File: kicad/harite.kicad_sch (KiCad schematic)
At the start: 77 parts, among them J1 503480-0500, J4 5034801200, J5 5034801200, U1 RP2040_Zero, U2 RP2040_Zero

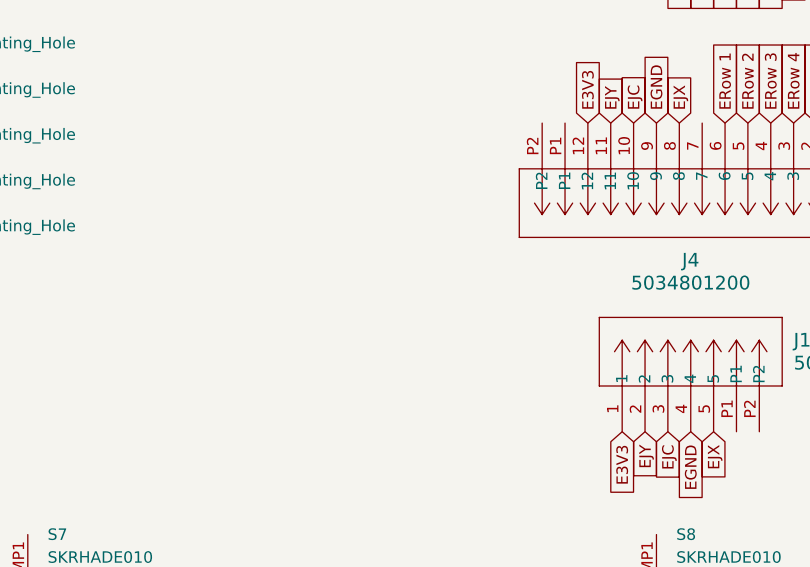
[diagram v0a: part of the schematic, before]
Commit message: update
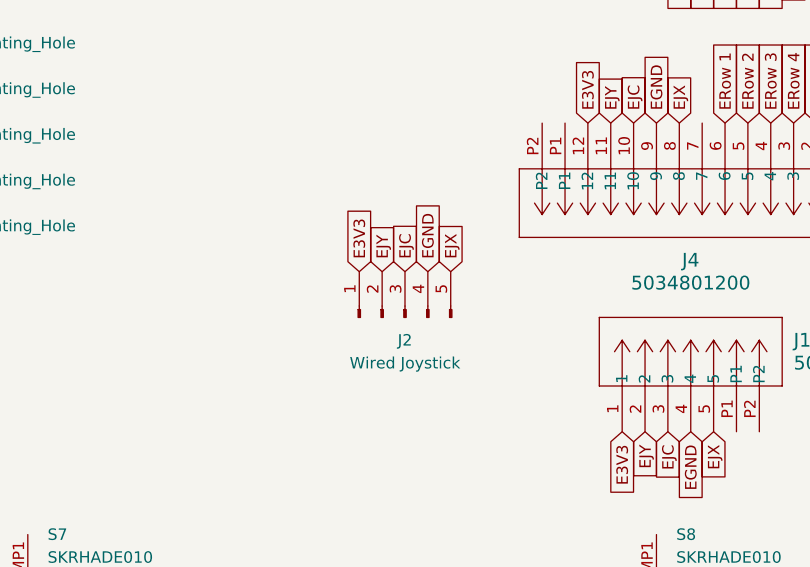
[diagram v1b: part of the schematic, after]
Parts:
- added J2: Wired Joystick, Wired-Joystick, symbol Connector:Conn_01x05_Pin
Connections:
- net E3V3: now also J2.1 (Pin_1)
- net EGND: now also J2.4 (Pin_4)
- net EJC: now also J2.3 (Pin_3)
- net EJX: now also J2.5 (Pin_5)
- net EJY: now also J2.2 (Pin_2)
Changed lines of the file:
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@@
 		)
 	)
+	(global_label "EJY"
+		(shape input)
+		(at 162.56 133.35 90)
+		(fields_autoplaced yes)
+		(effects
+			(font
+				(size 1.27 1.27)
+			)
+			(justify left)
+		)
+		(property "Intersheetrefs" "${INTERSHEET_REFS}"
+			(at 162.56 127.1596 90)
+			(effects
+				(font
+					(size 1.27 1.27)
+				)
+				(justify left)
+				(hide yes)
+			)
+		)
+	)
 	(global_label "RCol 3"
 		(shape input)
@@
 		)
 	)
+	(global_label "E3V3"
+		(shape input)
+		(at 160.02 133.35 90)
+		(fields_autoplaced yes)
+		(effects
+			(font
+				(size 1.27 1.27)
+			)
+			(justify left)
+		)
+		(property "Intersheetrefs" "${INTERSHEET_REFS}"
+			(at 160.02 125.7082 90)
+			(effects
+				(font
+					(size 1.27 1.27)
+				)
+				(justify left)
+				(hide yes)
+			)
+		)
+	)
 	(global_label "JX"
 		(shape input)
@@
 		)
 	)
+	(global_label "EJC"
+		(shape input)
+		(at 165.1 133.35 90)
+		(fields_autoplaced yes)
+		(effects
+			(font
+				(size 1.27 1.27)
+			)
+			(justify left)
+		)
+		(property "Intersheetrefs" "${INTERSHEET_REFS}"
+			(at 165.1 126.9782 90)
+			(effects
+				(font
+					(size 1.27 1.27)
+				)
+				(justify left)
+				(hide yes)
+			)
+		)
+	)
 	(global_label "JC"
 		(shape input)
@@
 		)
 	)
+	(global_label "EJX"
+		(shape input)
+		(at 170.18 133.35 90)
+		(fields_autoplaced yes)
+		(effects
+			(font
+				(size 1.27 1.27)
+			)
+			(justify left)
+		)
+		(property "Intersheetrefs" "${INTERSHEET_REFS}"
+			(at 170.18 127.0387 90)
+			(effects
+				(font
+					(size 1.27 1.27)
+				)
+				(justify left)
+				(hide yes)
+			)
+		)
+	)
 	(global_label "Col 3"
 		(shape input)
@@
 		)
 	)
+	(global_label "EGND"
+		(shape input)
+		(at 167.64 133.35 90)
+		(fields_autoplaced yes)
+		(effects
+			(font
+				(size 1.27 1.27)
+			)
+			(justify left)
+		)
+		(property "Intersheetrefs" "${INTERSHEET_REFS}"
+			(at 167.64 125.3453 90)
+			(effects
+				(font
+					(size 1.27 1.27)
+				)
+				(justify left)
+				(hide yes)
+			)
+		)
+	)
 	(global_label "Row 5"
 		(shape input)
@@
 					(unit 1)
 				)
+			)
+		)
+	)
+	(symbol
+		(lib_id "Connector:Conn_01x05_Pin")
+		(at 165.1 138.43 90)
+		(unit 1)
+		(exclude_from_sim no)
+		(in_bom yes)
+		(on_board yes)
+		(dnp no)
+		(fields_autoplaced yes)
+		(property "Reference" "J2"
+			(at 165.1 140.97 90)
+			(effects
+				(font
+					(size 1.27 1.27)
+				)
+			)
+		)
+		(property "Value" "Wired Joystick"
+			(at 165.1 143.51 90)
+			(effects
+				(font
+					(size 1.27 1.27)
+				)
+			)
+		)
+		(property "Footprint" "Wired-Joystick"
+			(at 165.1 138.43 0)
+			(effects
+				(font
+					(size 1.27 1.27)
+				)
+				(hide yes)
+			)
+		)
+		(property "Datasheet" "~"
+			(at 165.1 138.43 0)
+			(effects
+				(font
+					(size 1.27 1.27)
+				)
+				(hide yes)
+			)
+		)
+		(property "Description" "Generic connector, single row, 01x05, script generated"
+			(at 165.1 138.43 0)
+			(effects
+				(font
+					(size 1.27 1.27)
+				)
+				(hide yes)
+			)
+		)
+		(pin "4"
+		)
+		(pin "3"
+		)
+		(pin "2"
+		)
+		(pin "1"
+		)
+		(pin "5"
+		)
+		(instances
+			(project "harite"
+				(path "/feb70c3f-3e34-4f8f-9694-07d231f2d237"
+					(reference "J2")
+					(unit 1)
+				)

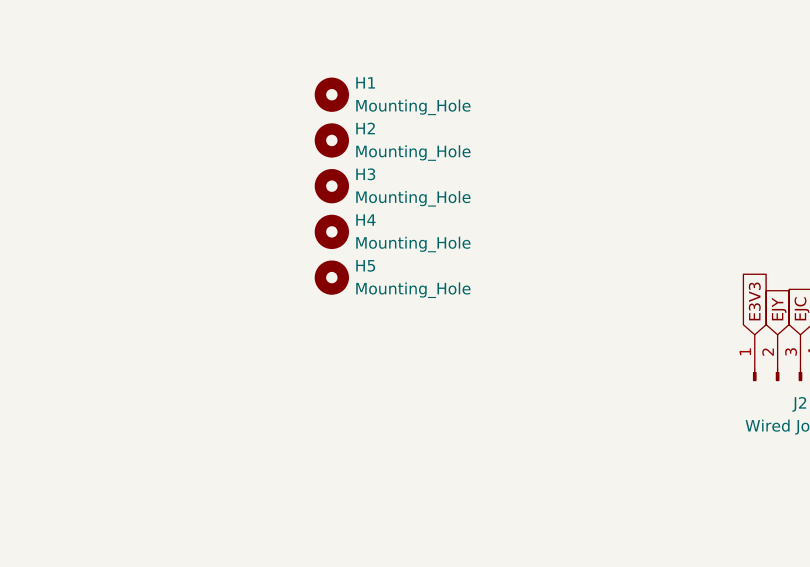
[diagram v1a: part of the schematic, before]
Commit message: add joycon
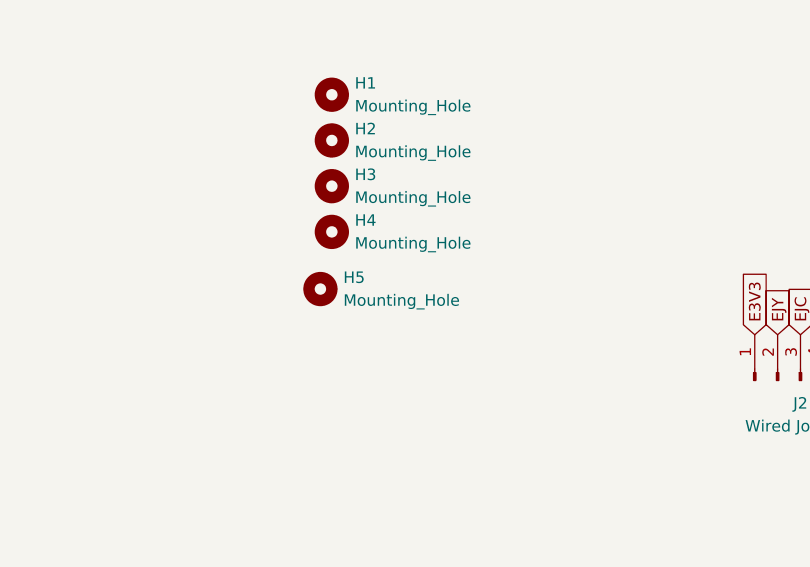
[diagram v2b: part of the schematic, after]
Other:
- moved on the sheet: H5
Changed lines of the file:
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@@
 	(symbol
 		(lib_id "ScottoKeebs:Placeholder_Mounting_Hole")
-		(at 113.03 127 0)
+		(at 111.76 128.27 0)
 		(unit 1)
 		(exclude_from_sim no)
@@
 		(fields_autoplaced yes)
 		(property "Reference" "H5"
-			(at 115.57 125.7299 0)
+			(at 114.3 126.9999 0)
 			(effects
 				(font
@@
 		)
 		(property "Value" "Mounting_Hole"
-			(at 115.57 128.2699 0)
+			(at 114.3 129.5399 0)
 			(effects
 				(font
@@
 		)
 		(property "Footprint" "MountingHole:MountingHole_2.2mm_M2_Pad_Via"
-			(at 113.03 127 0)
+			(at 111.76 128.27 0)
 			(effects
 				(font
@@
 		)
 		(property "Datasheet" "~"
-			(at 113.03 127 0)
+			(at 111.76 128.27 0)
 			(effects
 				(font
@@
 		)
 		(property "Description" "Mounting Hole without connection"
-			(at 113.03 127 0)
+			(at 111.76 128.27 0)
 			(effects
 				(font
@@
 	)
 	(symbol
-		(lib_id "ScottoKeebs:Placeholder_Mounting_Hole")
-		(at 120.65 243.84 0)
-		(unit 1)
-		(exclude_from_sim no)
-		(in_bom yes)
-		(on_board yes)
-		(dnp no)
-		(fields_autoplaced yes)
-		(property "Reference" "H9"
-			(at 123.19 242.5699 0)
-			(effects
-				(font
-					(size 1.27 1.27)
-				)
-				(justify left)
-			)
-		)
-		(property "Value" "Mounting_Hole"
-			(at 123.19 245.1099 0)
-			(effects
-				(font
-					(size 1.27 1.27)
-				)
-				(justify left)
-			)
-		)
-		(property "Footprint" "MountingHole:MountingHole_2.2mm_M2_Pad_Via"
-			(at 120.65 243.84 0)
-			(effects
-				(font
-					(size 1.27 1.27)
-				)
-				(hide yes)
-			)
-		)
-		(property "Datasheet" "~"
-			(at 120.65 243.84 0)
-			(effects
-				(font
-					(size 1.27 1.27)
-				)
-				(hide yes)
-			)
-		)
-		(property "Description" "Mounting Hole without connection"
-			(at 120.65 243.84 0)
-			(effects
-				(font
-					(size 1.27 1.27)
-				)
-				(hide yes)
-			)
-		)
-		(instances
-			(project "harite"
-				(path "/feb70c3f-3e34-4f8f-9694-07d231f2d237"
-					(reference "H9")
-					(unit 1)
-				)
-			)
-		)
-	)
-	(symbol
 		(lib_id "Device:D")
 		(at 163.83 60.96 0)
@@
 	)
 	(symbol
-		(lib_id "ScottoKeebs:Placeholder_Mounting_Hole")
-		(at 120.65 248.92 0)
-		(unit 1)
-		(exclude_from_sim no)
-		(in_bom yes)
-		(on_board yes)
-		(dnp no)
-		(fields_autoplaced yes)
-		(property "Reference" "H10"
-			(at 123.19 247.6499 0)
-			(effects
-				(font
-					(size 1.27 1.27)
-				)
-				(justify left)
-			)
-		)
-		(property "Value" "Mounting_Hole"
-			(at 123.19 250.1899 0)
-			(effects
-				(font
-					(size 1.27 1.27)
-				)
-				(justify left)
-			)
-		)
-		(property "Footprint" "MountingHole:MountingHole_2.2mm_M2_Pad_Via"
-			(at 120.65 248.92 0)
-			(effects
-				(font
-					(size 1.27 1.27)
-				)
-				(hide yes)
-			)
-		)
-		(property "Datasheet" "~"
-			(at 120.65 248.92 0)
-			(effects
-				(font
-					(size 1.27 1.27)
-				)
-				(hide yes)
-			)
-		)
-		(property "Description" "Mounting Hole without connection"
-			(at 120.65 248.92 0)
-			(effects
-				(font
-					(size 1.27 1.27)
-				)
-				(hide yes)
-			)
-		)
-		(instances
-			(project "harite"
-				(path "/feb70c3f-3e34-4f8f-9694-07d231f2d237"
-					(reference "H10")
-					(unit 1)
-				)
-			)
-		)
-	)
-	(symbol
 		(lib_id "Device:D")
 		(at 276.86 60.96 180)
@@
 	)
 	(symbol
+		(lib_id "ScottoKeebs:Placeholder_Mounting_Hole")
+		(at 120.65 243.84 0)
+		(unit 1)
+		(exclude_from_sim no)
+		(in_bom yes)
+		(on_board yes)
+		(dnp no)
+		(fields_autoplaced yes)
+		(property "Reference" "H9"
+			(at 123.19 242.5699 0)
+			(effects
+				(font
+					(size 1.27 1.27)
+				)
+				(justify left)
+			)
+		)
+		(property "Value" "Mounting_Hole"
+			(at 123.19 245.1099 0)
+			(effects
+				(font
+					(size 1.27 1.27)
+				)
+				(justify left)
+			)
+		)
+		(property "Footprint" "MountingHole:MountingHole_2.2mm_M2_Pad_Via"
+			(at 120.65 243.84 0)
+			(effects
+				(font
+					(size 1.27 1.27)
+				)
+				(hide yes)
+			)
+		)
+		(property "Datasheet" "~"
+			(at 120.65 243.84 0)
+			(effects
+				(font
+					(size 1.27 1.27)
+				)
+				(hide yes)
+			)
+		)
+		(property "Description" "Mounting Hole without connection"
+			(at 120.65 243.84 0)
+			(effects
+				(font
+					(size 1.27 1.27)
+				)
+				(hide yes)
+			)
+		)
+		(instances
+			(project "harite"
+				(path "/feb70c3f-3e34-4f8f-9694-07d231f2d237"
+					(reference "H9")
+					(unit 1)
+				)
+			)
+		)
+	)
+	(symbol
 		(lib_id "SKRHADE010:SKRHADE010")
 		(at 243.84 241.3 0)
@@
 					(unit 1)
 				)
+			)
+		)
+	)
+	(symbol
+		(lib_id "ScottoKeebs:Placeholder_Mounting_Hole")
+		(at 120.65 248.92 0)
+		(unit 1)
+		(exclude_from_sim no)
+		(in_bom yes)
+		(on_board yes)
+		(dnp no)
+		(fields_autoplaced yes)
+		(property "Reference" "H10"
+			(at 123.19 247.6499 0)
+			(effects
+				(font
+					(size 1.27 1.27)
+				)
+				(justify left)
+			)
+		)
+		(property "Value" "Mounting_Hole"
+			(at 123.19 250.1899 0)
+			(effects
+				(font
+					(size 1.27 1.27)
+				)
+				(justify left)
+			)
+		)
+		(property "Footprint" "MountingHole:MountingHole_2.2mm_M2_Pad_Via"
+			(at 120.65 248.92 0)
+			(effects
+				(font
+					(size 1.27 1.27)
+				)
+				(hide yes)
+			)
+		)
+		(property "Datasheet" "~"
+			(at 120.65 248.92 0)
+			(effects
+				(font
+					(size 1.27 1.27)
+				)
+				(hide yes)
+			)
+		)
+		(property "Description" "Mounting Hole without connection"
+			(at 120.65 248.92 0)
+			(effects
+				(font
+					(size 1.27 1.27)
+				)
+				(hide yes)
+			)
+		)
+		(instances
+			(project "harite"
+				(path "/feb70c3f-3e34-4f8f-9694-07d231f2d237"
+					(reference "H10")
+					(unit 1)
+				)
